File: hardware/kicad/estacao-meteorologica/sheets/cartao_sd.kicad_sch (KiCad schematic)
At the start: 7 parts, among them J17 Micro_SD_Card, U11 74LVC125

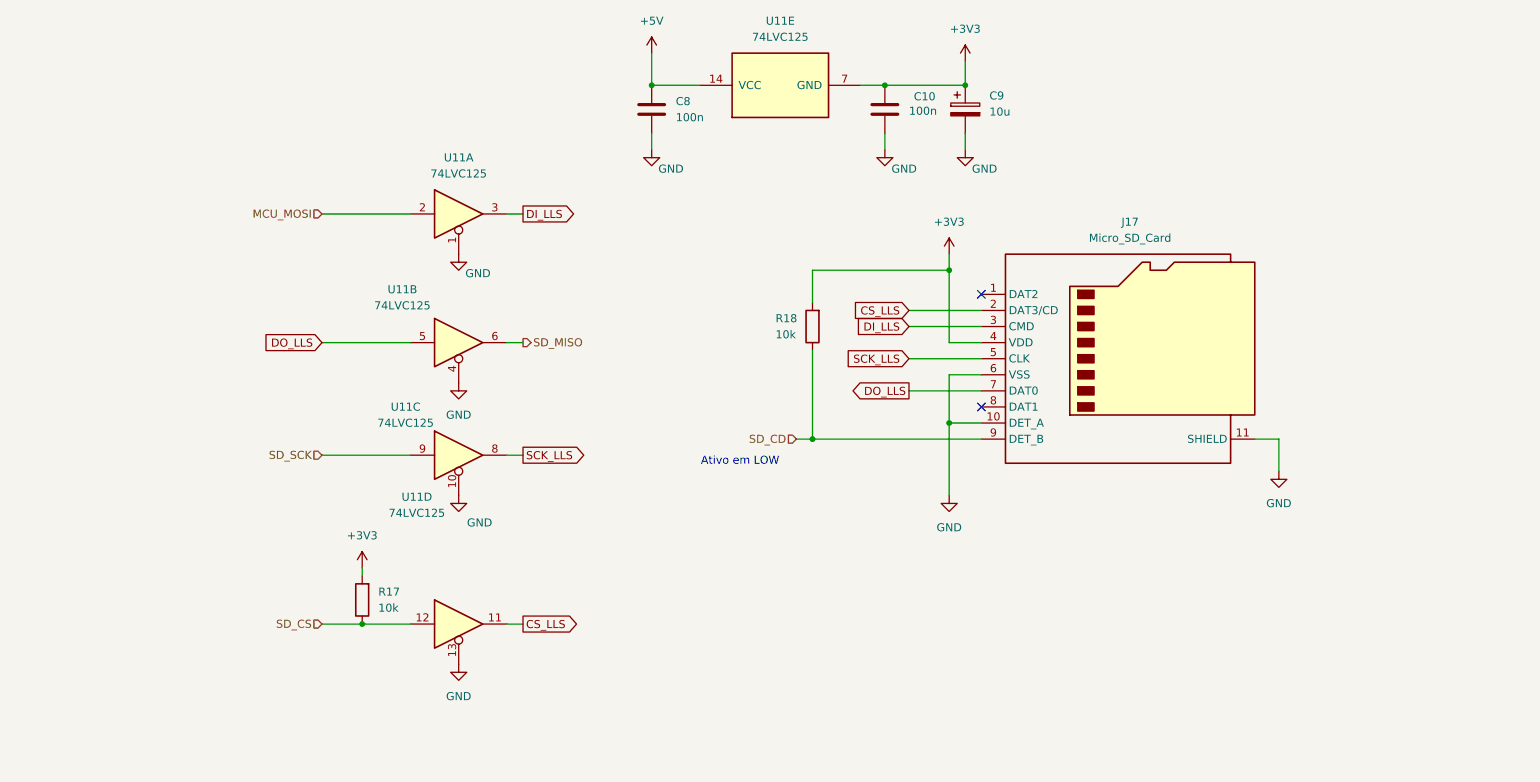
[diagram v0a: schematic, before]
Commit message: refatoracao: atualizacoes de hardware e falta revisao LoRa
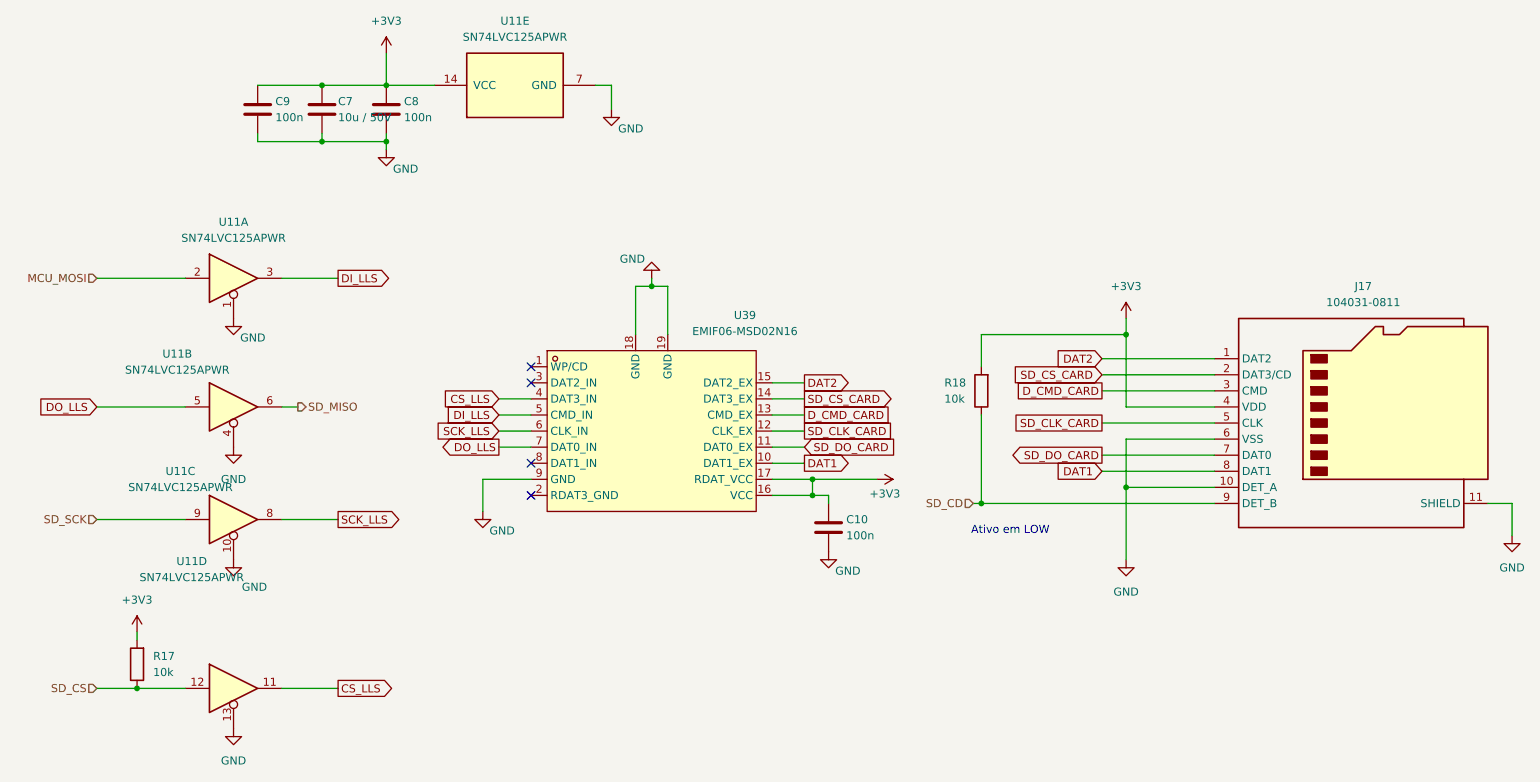
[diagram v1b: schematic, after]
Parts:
- removed C9: 10u, symbol Device:C_Polarized
- added C7: 10u / 50V, Capacitor_SMD:C_1206_3216Metric, symbol Device:C
- added C9: 100n, Capacitor_SMD:C_0603_1608Metric, symbol Device:C
- added U39: EMIF06-MSD02N16, Hardware_SD:QFN-16L_L3.5-W1.2-P0.40_EMIF06-MSD02N16, symbol Hardware_SD:EMIF06-MSD02N16
- C10, C8: footprint (none) -> Capacitor_SMD:C_0603_1608Metric; LCSC (none) -> C14663; LCSC Part (none) -> C14663; MPN (none) -> CC0603KRX7R9BB104; Manufacturer (none) -> YAGEO; Rating (none) -> X7R; 100 nF; 50 V; ±10 %; 0603
- J17: value Micro_SD_Card -> 104031-0811; MPN (none) -> 104031-0811; Manufacturer (none) -> Molex; Rating (none) -> 10 V; 0.5 A; -25 °C to +85 °C; SMT
- R17, R18: footprint (none) -> Resistor_SMD:R_0603_1608Metric; LCSC (none) -> C25804; LCSC Part (none) -> C25804; MPN (none) -> 0603WAF1002T5E; Manufacturer (none) -> UNI-ROYAL; Rating (none) -> 10 kOhm; ±1 %; 0.1 W; 0603
- U11: value 74LVC125 -> SN74LVC125APWR; LCSC (none) -> C7813; LCSC Part (none) -> C7813; MPN (none) -> SN74LVC125APWR; Manufacturer (none) -> Texas Instruments; Rating (none) -> VCC 1.65 V to 3.6 V; 24 mA; TSSOP-14
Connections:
- net +5V is gone; now on net +3V3: C8.1, U11.14 (VCC)
- net +3V3: now also C7.1, C9.1, U39.16 (VCC), U39.17 (RDAT_VCC); no longer U11.7 (GND)
- net CS_LLS: now also U39.4 (DAT3_IN); no longer J17.2 (DAT3/CD)
- net DI_LLS: now also U39.5 (CMD_IN); no longer J17.3 (CMD)
- net DO_LLS: now also U39.7 (DAT0_IN); no longer J17.7 (DAT0)
- net GND: now also U11.7 (GND), C7.2, C9.2, U39.18 (GND), U39.19 (GND), U39.9 (GND)
- net SCK_LLS: now also U39.6 (CLK_IN); no longer J17.5 (CLK)
- net DAT2: now reaches J17.1 (DAT2)
- net DAT2: now also U39.15 (DAT2_EX)
- net DAT1: now reaches J17.8 (DAT1)
- net DAT1: now also U39.10 (DAT1_EX)
- new net D_CMD_CARD: J17.3 (CMD), U39.13 (CMD_EX)
- new net SD_CLK_CARD: J17.5 (CLK), U39.12 (CLK_EX)
- new net SD_CS_CARD: J17.2 (DAT3/CD), U39.14 (DAT3_EX)
- new net SD_DO_CARD: J17.7 (DAT0), U39.11 (DAT0_EX)
- no-connect marks 2 -> 4
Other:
- moved on the sheet: C8, J17, R17, R18, U11A, U11B, U11C, U11D, U11E
